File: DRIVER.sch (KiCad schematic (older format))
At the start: 24 parts, among them P1 PWR_IN, P2 HALL, P3 MOT, U1 MCT8316ZR

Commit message: Update
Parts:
- added D1: ORANGE, symbol device:LED
- added D2: BLUE, symbol device:LED
- added D3: GREEN, symbol device:LED
- added D4: RED, symbol device:LED
- added R1, R2: 1k, Resistor_SMD:R_0603_1608Metric, symbol device:R
- added R3: 4.7k, Resistor_SMD:R_0402_1005Metric, symbol device:R
- added R4: 330, Resistor_SMD:R_0402_1005Metric, symbol device:R
- R10: renamed from R6; value 10k 1% 1/16W -> 10k
- R12: renamed from R8; value 10k 1% 1/16W -> 10k
- R7: renamed from R3; value 10k 1% 1/16W -> 10k
- renumbered R7 to R11, R9 to R13, R1 to R5, R2 to R6, R4 to R8, R5 to R9
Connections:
- net labels added: +3.3V, +5V
- net labels removed: VCC, VDD
- wire segments 150 -> 167

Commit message: Update
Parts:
- C1: symbol device:CP1 -> Driverino-rescue:CP1-device
- C10, C2, C3, C4, C5, C6, C7, C8, C9: symbol device:C -> Driverino-rescue:C-device
- D1, D2, D3, D4: symbol device:LED -> Driverino-rescue:LED-device
- L1: symbol device:INDUCTOR_SMALL -> Driverino-rescue:INDUCTOR_SMALL-device
- P1: symbol conn:CONN_2 -> Driverino-rescue:CONN_2-conn
- P2: symbol conn:CONN_8 -> Driverino-rescue:CONN_8-conn
- P3: symbol conn:CONN_3 -> Driverino-rescue:CONN_3-conn
- R1, R10, R11, R12, R13, R2, R3, R4, R5, R6, R7, R8, R9: symbol device:R -> Driverino-rescue:R-device
- U1: symbol texas2:MCT8316Z -> Driverino-rescue:MCT8316Z-texas2
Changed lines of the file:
@@
 W
 $Comp
-L device:C C?
+L Driverino-rescue:C-device C?
 U 1 1 613F2407
 P 7025 4250
@@
 $EndComp
 $Comp
-L device:C C?
+L Driverino-rescue:C-device C?
 U 1 1 613F240F
 P 7025 3725
@@
 HBP
 $Comp
-L device:C C?
+L Driverino-rescue:C-device C?
 U 1 1 613F2422
 P 2250 4275
@@
 $EndComp
 $Comp
-L power:GNDPWR #PWR?
+L Driverino-rescue:GNDPWR-power #PWR?
 U 1 1 613F2428
 P 4500 5625
@@
 	6050 3600 6050 4450
 $Comp
-L device:C C?
+L Driverino-rescue:C-device C?
 U 1 1 613F2449
 P 3250 3600
@@
 	5875 3700 5875 2650
 $Comp
-L device:C C?
+L Driverino-rescue:C-device C?
 U 1 1 613F2468
 P 5875 4000
@@
 	5875 4200 5875 4450
 $Comp
-L power:GND #PWR?
+L Driverino-rescue:GND-power #PWR?
 U 1 1 613F2471
 P 5875 4650
@@
 	5500 3900 5500 4800
 $Comp
-L device:R R?
+L Driverino-rescue:R-device R?
 U 1 1 613F2482
 P 4000 1925
@@
 	4000 1575 4000 1675
 $Comp
-L device:C C?
+L Driverino-rescue:C-device C?
 U 1 1 613F2491
 P 2650 4275
@@
 	6675 3400 7025 3400
 $Comp
-L device:C C?
+L Driverino-rescue:C-device C?
 U 1 1 613F24A8
 P 7025 3200
@@
 	2250 3550 2250 3700
 $Comp
-L device:C C?
+L Driverino-rescue:C-device C?
 U 1 1 613F24BD
 P 2650 3700
@@
 Connection ~ 4700 2350
 $Comp
-L device:R R?
+L Driverino-rescue:R-device R?
 U 1 1 613F24EA
 P 4700 1925
@@
 	10325 5675 9950 5675
 $Comp
-L conn:CONN_3 P?
+L Driverino-rescue:CONN_3-conn P?
 U 1 1 614094B0
 P 10675 5575
@@
 	9375 3875 9125 3875
 $Comp
-L device:R R?
+L Driverino-rescue:R-device R?
 U 1 1 614094E1
 P 9375 4200
@@
 $EndComp
 $Comp
-L device:R R?
+L Driverino-rescue:R-device R?
 U 1 1 614094E7
 P 9550 4200
@@
 $EndComp
 $Comp
-L device:R R?
+L Driverino-rescue:R-device R?
 U 1 1 614094ED
 P 9725 4200
@@
 	9725 3375 9125 3375
 $Comp
-L device:R R?
+L Driverino-rescue:R-device R?
 U 1 1 61409506
 P 9725 3025
@@
 $EndComp
 $Comp
-L device:R R?
+L Driverino-rescue:R-device R?
 U 1 1 61409516
 P 9550 3025
@@
 $EndComp
 $Comp
-L device:R R?
+L Driverino-rescue:R-device R?
 U 1 1 61409526
 P 9375 3025
@@
 	9675 1100 9975 1100
 $Comp
-L conn:CONN_2 P?
+L Driverino-rescue:CONN_2-conn P?
 U 1 1 614328C9
 P 10675 1200
@@
 	9975 1100 10325 1100
 $Comp
-L power:GNDPWR #PWR?
+L Driverino-rescue:GNDPWR-power #PWR?
 U 1 1 614328D8
 P 9975 1500
@@
 Connection ~ 9975 1300
 $Comp
-L device:R R?
+L Driverino-rescue:R-device R?
 U 1 1 614328E5
 P 9500 1300
@@
 	9075 1300 9075 1500
 $Comp
-L power:GND #PWR?
+L Driverino-rescue:GND-power #PWR?
 U 1 1 614328EC
 P 9075 1500
@@
 MISO
 $Comp
-L device:INDUCTOR_SMALL L?
+L Driverino-rescue:INDUCTOR_SMALL-device L?
 U 1 1 6145D79B
 P 4625 6450
@@
 $EndComp
 $Comp
-L device:C C?
+L Driverino-rescue:C-device C?
 U 1 1 6145D7A1
-P 4200 6775
+P 4200 6750
 AR Path="/6145D7A1" Ref="C?"  Part="1"
 AR Path="/613CDDB7/6145D7A1" Ref="C6"  Part="1"
-F 0 "C6" H 4075 6725 40  0000 R CNN
-F 1 "22uF" H 4075 6775 40  0000 R CNN
-F 2 "" H 4238 6625 30  0000 C CNN
-F 3 "" H 4200 6775 60  0000 C CNN
-	1    4200 6775
+F 0 "C6" H 4075 6700 40  0000 R CNN
+F 1 "22uF" H 4075 6750 40  0000 R CNN
+F 2 "" H 4238 6600 30  0000 C CNN
+F 3 "" H 4200 6750 60  0000 C CNN
+	1    4200 6750
 	-1   0    0    1
 $EndComp
@@
 	4375 6450 4200 6450
 Wire Wire Line
-	4200 6450 4200 6575
-$Comp
-L power:GND #PWR?
+	4200 6450 4200 6550
+$Comp
+L Driverino-rescue:GND-power #PWR?
 U 1 1 6145D7AB
 P 4200 7125
@@
 $EndComp
 Wire Wire Line
-	4200 6975 4200 7050
+	4200 6950 4200 7050
 Wire Wire Line
 	4200 7050 5050 7050
@@
 	1625 4475 1625 4550
 $Comp
-L power:GNDPWR #PWR?
+L Driverino-rescue:GNDPWR-power #PWR?
 U 1 1 613F24DF
 P 1625 4650
@@
 	2250 4000 1625 4000
 $Comp
-L device:CP1 C?
+L Driverino-rescue:CP1-device C?
 U 1 1 613F24D7
 P 1625 4275
@@
 $EndComp
 $Comp
-L power:+5V #PWR012
+L Driverino-rescue:+5V-power #PWR012
 U 1 1 608D548F
 P 4200 6200
@@
 $EndComp
 $Comp
-L power:+3.3V #PWR016
+L Driverino-rescue:+3.3V-power #PWR016
 U 1 1 608D6090
 P 5875 2650
@@
 $EndComp
 $Comp
-L power:+3.3V #PWR011
+L Driverino-rescue:+3.3V-power #PWR011
 U 1 1 608E3D65
 P 4000 1575
@@
 $EndComp
 $Comp
-L power:+3.3V #PWR015
+L Driverino-rescue:+3.3V-power #PWR015
 U 1 1 608E3F5E
 P 4700 1575
@@
 	4000 2325 4000 2450
 $Comp
-L texas2:MCT8316Z U?
+L Driverino-rescue:MCT8316Z-texas2 U?
 U 1 1 613F23CB
 P 4350 3550
@@
 	2950 2750 2700 2750
 $Comp
-L power:GND #PWR?
+L Driverino-rescue:GND-power #PWR?
 U 1 1 613F23E8
 P 2700 2750
@@
 Connection ~ 2950 2750
 $Comp
-L power:+3.3V #PWR021
+L Driverino-rescue:+3.3V-power #PWR021
 U 1 1 609B9EEF
 P 9975 2550
@@
 	10325 3875 9375 3875
 $Comp
-L conn:CONN_8 P?
+L Driverino-rescue:CONN_8-conn P?
 U 1 1 614094BA
 P 10675 3625
@@
 	10325 3975 9975 3975
 $Comp
-L power:GND #PWR?
+L Driverino-rescue:GND-power #PWR?
 U 1 1 614094C1
 P 9975 4700
@@
 $EndComp
 $Comp
-L device:R R?
+L Driverino-rescue:R-device R?
 U 1 1 60AF5785
 P 2025 6600
@@
 $EndComp
 $Comp
-L power:GNDPWR #PWR?
+L Driverino-rescue:GNDPWR-power #PWR?
 U 1 1 60AF5F0E
 P 2025 7425
@@
 	2025 6850 2025 6900
 $Comp
-L device:LED D3
+L Driverino-rescue:LED-device D3
 U 1 1 60B03561
 P 2025 7100
@@
 	2025 7300 2025 7425
 $Comp
-L device:R R?
+L Driverino-rescue:R-device R?
 U 1 1 60B112DD
 P 2425 6600
@@
 	2425 6850 2425 6900
 $Comp
-L device:LED D4
+L Driverino-rescue:LED-device D4
 U 1 1 60B112F3
 P 2425 7100
@@
 	2425 7300 2425 7425
 $Comp
-L power:+3.3V #PWR09
+L Driverino-rescue:+3.3V-power #PWR09
 U 1 1 60B18E8B
 P 2425 6200
@@
 	2425 6200 2425 6350
 $Comp
-L device:R R?
+L Driverino-rescue:R-device R?
 U 1 1 60B5A3E5
 P 1525 6600
@@
 	1525 7300 1525 7425
 $Comp
-L power:GND #PWR?
+L Driverino-rescue:GND-power #PWR?
 U 1 1 60B5A3ED
 P 1525 7425
@@
 $EndComp
 $Comp
-L device:LED D?
+L Driverino-rescue:LED-device D?
 U 1 1 60B5A3F3
 P 1525 7100
@@
 	1525 6850 1525 6900
 $Comp
-L power:+5V #PWR?
+L Driverino-rescue:+5V-power #PWR?
 U 1 1 60B5A3FA
 P 1525 6200
@@
 $EndComp
 $Comp
-L device:R R?
+L Driverino-rescue:R-device R?
 U 1 1 60B5A406
 P 1050 6600
@@
 	1050 7300 1050 7425
 $Comp
-L power:GND #PWR?
+L Driverino-rescue:GND-power #PWR?
 U 1 1 60B5A40E
 P 1050 7425
@@
 $EndComp
 $Comp
-L device:LED D?
+L Driverino-rescue:LED-device D?
 U 1 1 60B5A414
 P 1050 7100
@@
 	1050 6850 1050 6900
 $Comp
-L power:+3.3V #PWR?
+L Driverino-rescue:+3.3V-power #PWR?
 U 1 1 60B5A41B
 P 1050 6200

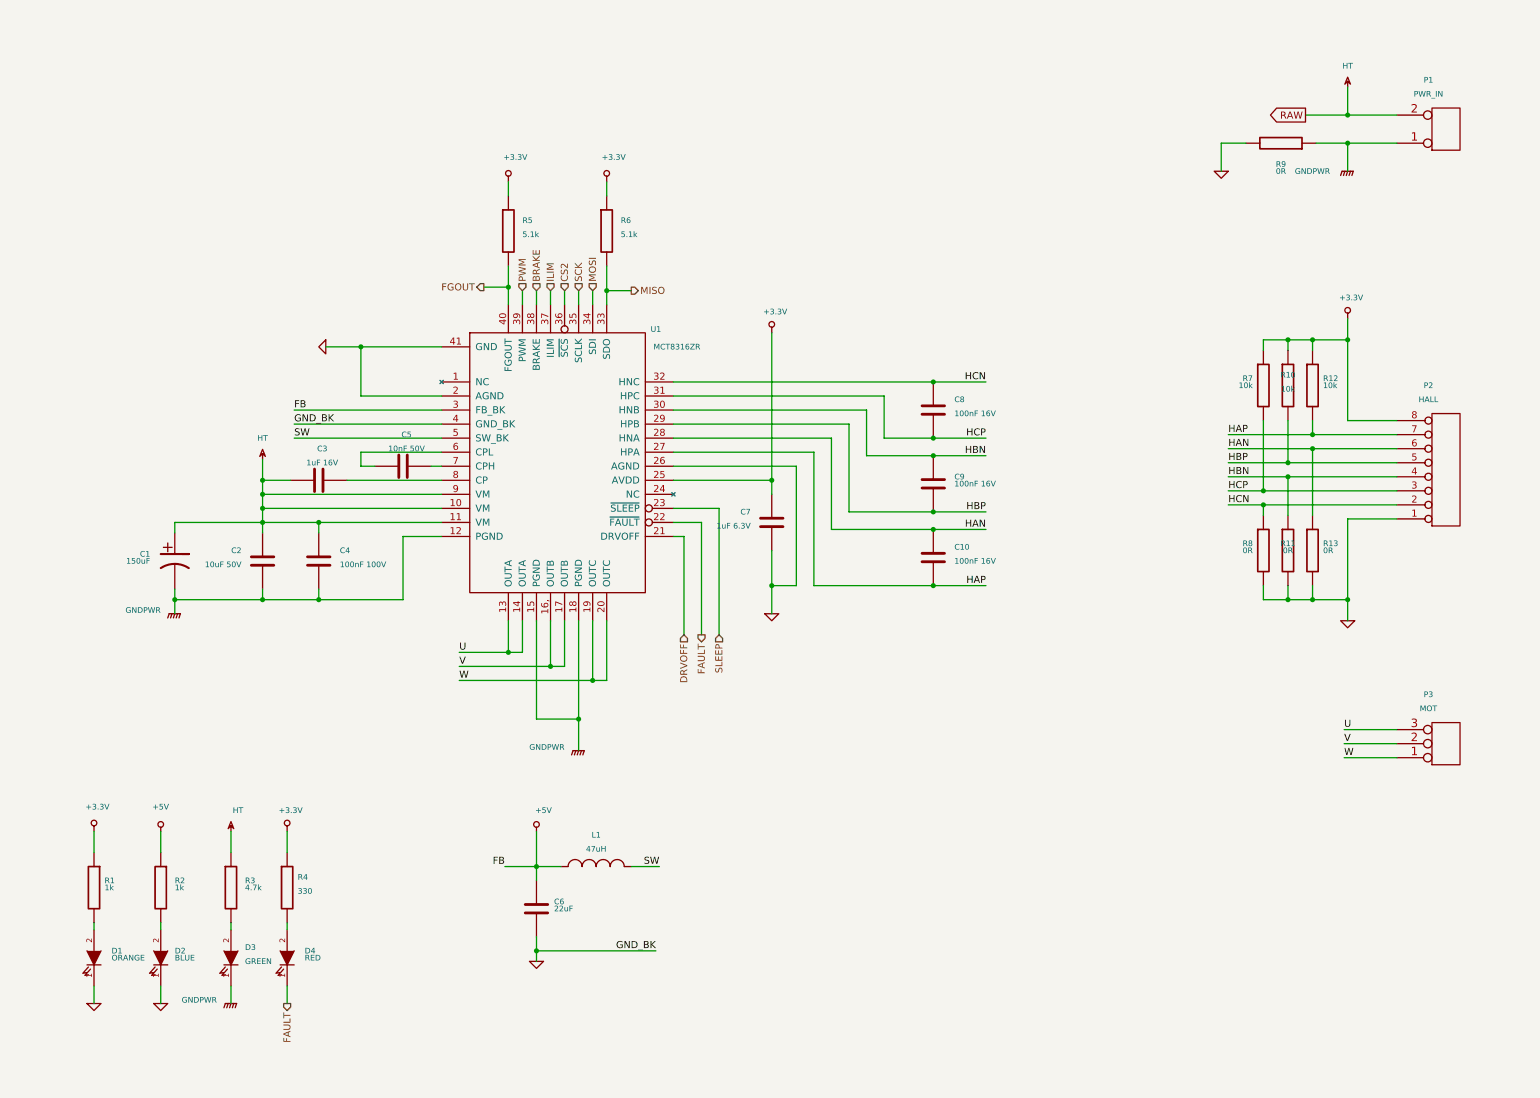
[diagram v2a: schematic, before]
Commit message: Update
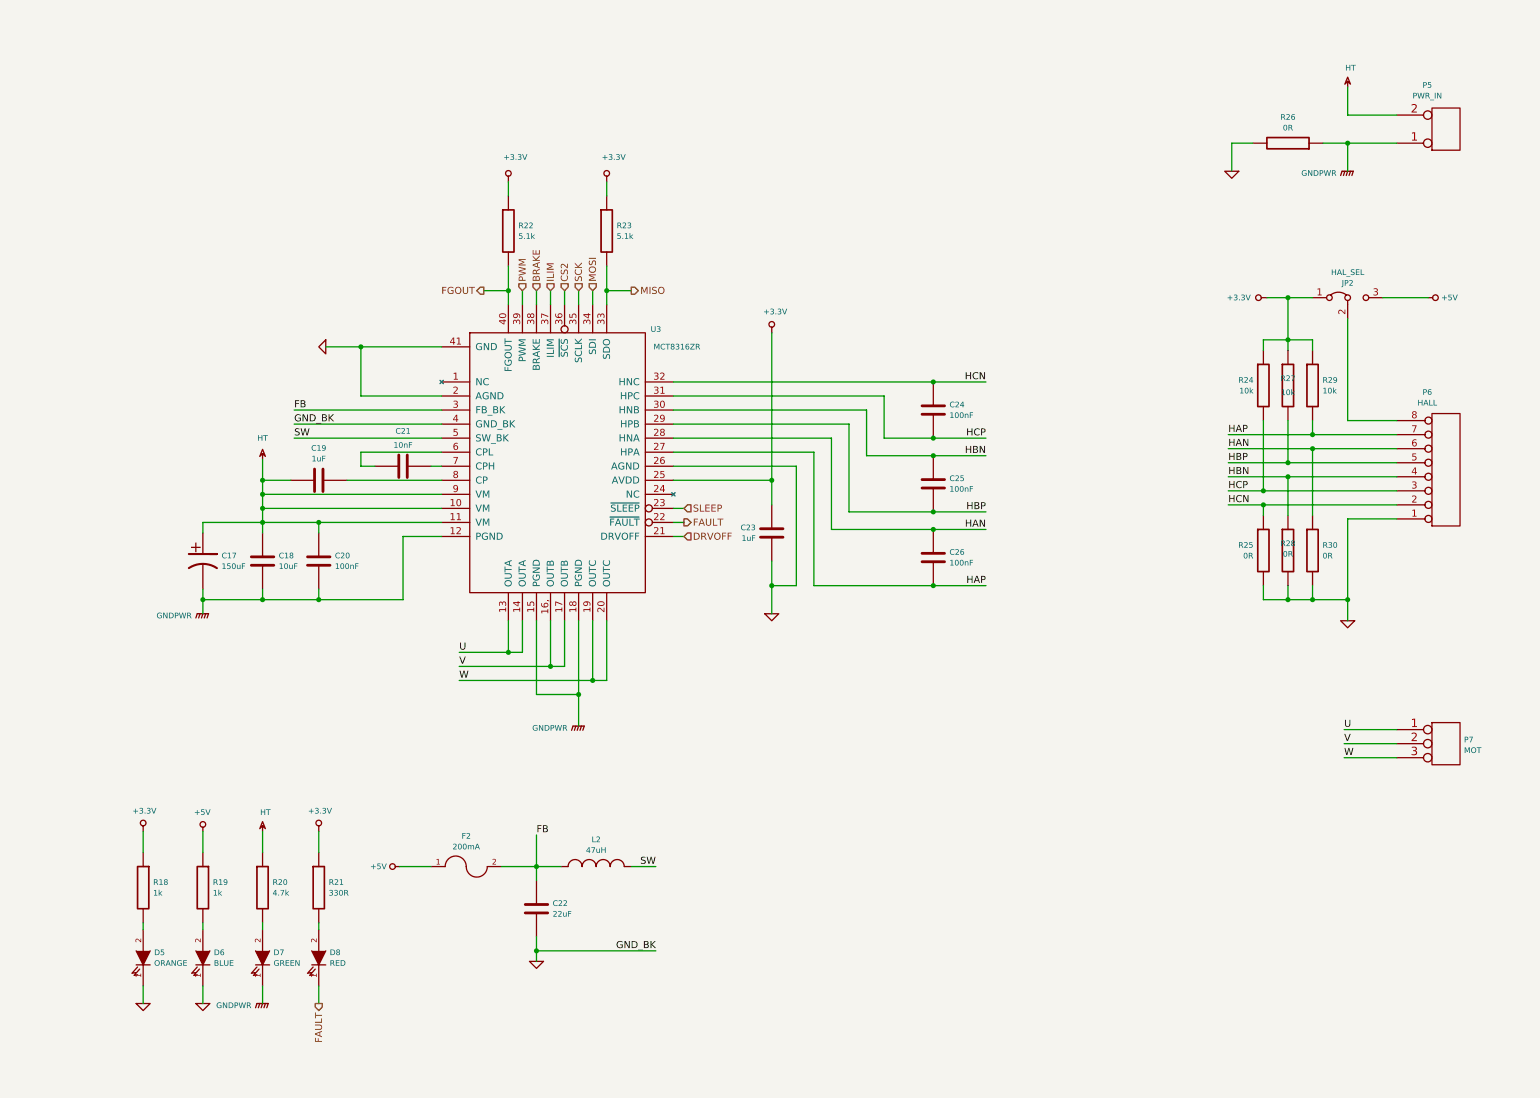
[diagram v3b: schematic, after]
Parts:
- added F2: 200mA, Fuse:Fuse_0402_1005Metric, symbol Driverino-rescue:FUSE-device
- added JP2: HAL_SEL, Driverino:TDD01H0SB1R, symbol Jumper:Jumper_3_Bridged12
- C17: renamed from C1; footprint (none) -> Capacitor_SMD:CP_Elec_6.3x7.7; P/N EEE-FTV151XAV -> (none); Productor Panasonic -> (none); Provider (none) -> Mouser; ProviderCode (none) -> 667-EEE-FTV151XAV
- C18: renamed from C2; value 10uF 50V -> 10uF; footprint Capacitor_SMD:C_0603_1608Metric -> Capacitor_SMD:C_1206_3216Metric; Manufacturer (none) -> TDK; Provider (none) -> Mouser; ProviderCode (none) -> 810-C3216X7R1H106160; manf# (none) -> C3216X7R1H106K160AE
- C19: renamed from C3; value 1uF 16V -> 1uF; Manufacturer (none) -> AVX; Provider (none) -> Mouser; ProviderCode (none) -> 581-0603DC105MAT2A; manf# (none) -> 0603DC105MAT2A
- C20: renamed from C4; value 100nF 100V -> 100nF; footprint Capacitor_SMD:C_0603_1608Metric -> Capacitor_SMD:C_0402_1005Metric; Manufacturer (none) -> Murata; Provider (none) -> Mouser; ProviderCode (none) -> 81-GCM155R71H104KE2J; manf# (none) -> GCM155R71H104KE02J
- C21: renamed from C5; value 10nF 50V -> 10nF; footprint Capacitor_SMD:C_0603_1608Metric -> Capacitor_SMD:C_0402_1005Metric; Manufacturer (none) -> Murata; Provider (none) -> Mouser; ProviderCode (none) -> 81-GRM155R71H103JA8D; manf# (none) -> GRM155R71H103JA88D
- C22: renamed from C6; footprint (none) -> Capacitor_SMD:C_1206_3216Metric; Manufacturer (none) -> Murata; Provider (none) -> Mouser; ProviderCode (none) -> 81-GCM31CR70J226KE3L; manf# (none) -> GCM31CR70J226KE23L
- C23: renamed from C7; value 1uF 6.3V -> 1uF; Manufacturer (none) -> AVX; Provider (none) -> Mouser; ProviderCode (none) -> 581-0603DC105MAT2A; manf# (none) -> 0603DC105MAT2A
- C24: renamed from C8; value 100nF 16V -> 100nF; footprint Capacitor_SMD:C_0603_1608Metric -> Capacitor_SMD:C_0402_1005Metric; Manufacturer (none) -> Murata; Provider (none) -> Mouser; ProviderCode (none) -> 81-GCM155R71H104KE2J; manf# (none) -> GCM155R71H104KE02J
- C25: renamed from C9; value 100nF 16V -> 100nF; footprint Capacitor_SMD:C_0603_1608Metric -> Capacitor_SMD:C_0402_1005Metric; Manufacturer (none) -> Murata; Provider (none) -> Mouser; ProviderCode (none) -> 81-GCM155R71H104KE2J; manf# (none) -> GCM155R71H104KE02J
- C26: renamed from C10; value 100nF 16V -> 100nF; footprint Capacitor_SMD:C_0603_1608Metric -> Capacitor_SMD:C_0402_1005Metric; Manufacturer (none) -> Murata; Provider (none) -> Mouser; ProviderCode (none) -> 81-GCM155R71H104KE2J; manf# (none) -> GCM155R71H104KE02J
- D5: renamed from D1; footprint (none) -> LED_SMD:LED_0603_1608Metric; Manufacturer (none) -> Kingbright; Provider (none) -> Mouser; ProviderCode (none) -> 604-AP1608SECK; manf# (none) -> AP1608SECK
- D6: renamed from D2; footprint (none) -> LED_SMD:LED_0603_1608Metric; Manufacturer (none) -> Kingbright; Provider (none) -> Mouser; ProviderCode (none) -> 604-APT1608QBC/D; manf# (none) -> APT1608QBC/D
- D7: renamed from D3; footprint (none) -> LED_SMD:LED_0603_1608Metric; Manufacturer (none) -> Kingbright; Provider (none) -> Mouser; ProviderCode (none) -> 604-APT1608SGC; manf# (none) -> APT1608SGC
- D8: renamed from D4; footprint (none) -> LED_SMD:LED_0603_1608Metric; Manufacturer (none) -> Kingbright; Provider (none) -> Mouser; ProviderCode (none) -> 604-APT1608EC; manf# (none) -> APT1608EC
- L2: renamed from L1; footprint (none) -> Inductor_SMD:L_1210_3225Metric; Manufacturer (none) -> Taiyo Yuden; Provider (none) -> Mouser; ProviderCode (none) -> 963-CBC3225T470KRV; manf# (none) -> CBC3225T470KRV
- P5: renamed from P1; footprint (none) -> Driverino:39773-0002; P/N 397730002 -> (none); Productor Molex -> (none); Provider (none) -> Mouser; ProviderCode (none) -> 538-39773-0002; manf# 397730002 -> 39773-0002
- P6: renamed from P2; footprint Connector_Molex:Molex_PicoBlade_53047-0810_1x03_P1.25mm_Vertical -> Connector_Molex:Molex_PicoBlade_53047-0810_1x08_P1.25mm_Vertical; Productor Molex -> (none); Provider (none) -> Mouser; ProviderCode (none) -> 538-53047-0810
- P7: renamed from P3; footprint (none) -> Driverino:39773-0003; P/N 397730003 -> (none); Productor Molex -> (none); Provider (none) -> Mouser; ProviderCode (none) -> 538-39773-0003; manf# 397730003 -> 39773-0003
- R18: renamed from R1; footprint Resistor_SMD:R_0603_1608Metric -> Resistor_SMD:R_0402_1005Metric; Manufacturer (none) -> Vishay; P/N CRCW0603332RFKEA -> (none); Productor Vishay -> (none); Provider (none) -> Mouser; ProviderCode (none) -> 71-CRCW04021K00FKEDC; manf# (none) -> CRCW04021K00FKEDC
- R19: renamed from R2; footprint Resistor_SMD:R_0603_1608Metric -> Resistor_SMD:R_0402_1005Metric; Manufacturer (none) -> Vishay; P/N CRCW0603332RFKEA -> (none); Productor Vishay -> (none); Provider (none) -> Mouser; ProviderCode (none) -> 71-CRCW04021K00FKEDC; manf# (none) -> CRCW04021K00FKEDC
- R20: renamed from R3; Manufacturer (none) -> Yageo; Productor TE Connectivity -> (none); Provider (none) -> Mouser; ProviderCode (none) -> 603-RC0402FR-074K7L; manf# (none) -> RC0402FR-074K7L
- R21: renamed from R4; value 330 -> 330R; Manufacturer (none) -> Vishay; Productor TE Connectivity -> (none); Provider (none) -> Mouser; ProviderCode (none) -> 756-GWCR0402330RFT10; manf# (none) -> CRCW0402330RFKED
- R22: renamed from R5; Manufacturer (none) -> ROHM; Provider (none) -> Mouser; ProviderCode (none) -> 755-SFR01MZPF5101; manf# (none) -> SFR01MZPF5101
- R23: renamed from R6; Manufacturer (none) -> ROHM; Provider (none) -> Mouser; ProviderCode (none) -> 755-SFR01MZPF5101; manf# (none) -> SFR01MZPF5101
- R24: renamed from R7; Manufacturer (none) -> Vishay; Productor TE Connectivity -> (none); Provider (none) -> Mouser; ProviderCode (none) -> 71-CRCW040210K0FKEDC; manf# (none) -> CRCW040210K0FKEDC
- R25: renamed from R8; footprint Resistor_SMD:R_0603_1608Metric -> Resistor_SMD:R_0402_1005Metric; Manufacturer (none) -> Vishay; Provider (none) -> Mouser; ProviderCode (none) -> 71-RCC04020000Z0ED; manf# (none) -> RCC04020000Z0ED
- R26: renamed from R9; footprint Resistor_SMD:R_0603_1608Metric -> Resistor_SMD:R_0402_1005Metric; Manufacturer (none) -> Vishay; P/N ERJU03F22R0V -> (none); Provider (none) -> Mouser; ProviderCode (none) -> 71-RCC04020000Z0ED; manf# (none) -> RCC04020000Z0ED
- R27: renamed from R10; Manufacturer (none) -> Vishay; Productor TE Connectivity -> (none); Provider (none) -> Mouser; ProviderCode (none) -> 71-CRCW040210K0FKEDC; manf# (none) -> CRCW040210K0FKEDC
- R28: renamed from R11; footprint Resistor_SMD:R_0603_1608Metric -> Resistor_SMD:R_0402_1005Metric; Manufacturer (none) -> Vishay; Provider (none) -> Mouser; ProviderCode (none) -> 71-RCC04020000Z0ED; manf# (none) -> RCC04020000Z0ED
- R29: renamed from R12; Manufacturer (none) -> Vishay; Productor TE Connectivity -> (none); Provider (none) -> Mouser; ProviderCode (none) -> 71-CRCW040210K0FKEDC; manf# (none) -> CRCW040210K0FKEDC
- R30: renamed from R13; footprint Resistor_SMD:R_0603_1608Metric -> Resistor_SMD:R_0402_1005Metric; Manufacturer (none) -> Vishay; Provider (none) -> Mouser; ProviderCode (none) -> 71-RCC04020000Z0ED; manf# (none) -> RCC04020000Z0ED
- U3: renamed from U1; footprint (none) -> Driverino:QFN-40_EP_5x7_Pitch0.5mm; Productor TI -> (none)
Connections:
- net +3.3V: now also JP2.1 (A); no longer P6.8 (P8)
- net +5V: now also F2.1, JP2.3 (B); no longer C22.2, L2.2, U3.3 (FB_BK)
- net U: now also P7.1 (P1); no longer P7.3 (P3)
- net W: now also P7.3 (P3); no longer P7.1 (P1)
- new net: JP2.2 (C), P6.8 (P8)
- new net FB: C22.2, F2.2, L2.2, U3.3 (FB_BK)
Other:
- moved on the sheet: C17, C23, D5, D6, D7, D8, R18, R19, R20, R21, R26

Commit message: Update
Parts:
- JP2: symbol Jumper:Jumper_3_Bridged12 -> Driverino-rescue:Jumper_3_Bridged12-Jumper
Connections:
- net GNDPWR: now also P5.2 (PM); no longer P5.1 (P1)
- net HT: now also P5.1 (P1); no longer P5.2 (PM)
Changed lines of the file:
@@
 AR Path="/614328C9" Ref="P?"  Part="1"
 AR Path="/613CDDB7/614328C9" Ref="P5"  Part="1"
-F 0 "P5" H 10542 887 40  0000 C CNN
-F 1 "PWR_IN" H 10542 963 40  0000 C CNN
+F 0 "P5" H 10850 1250 40  0000 L CNN
+F 1 "PWR_IN" H 10850 1150 40  0000 L CNN
 F 2 "Driverino:39773-0002" H 10675 1200 50  0001 C CNN
 F 3 "" H 10675 1200 50  0001 C CNN
@@
 F 9 "538-39773-0002" H 10675 1200 50  0001 C CNN "ProviderCode"
 	1    10675 1200
-	1    0    0    1
+	1    0    0    -1
 $EndComp
 $Comp
@@
 $EndComp
 $Comp
-L Jumper:Jumper_3_Bridged12 JP?
+L Driverino-rescue:Jumper_3_Bridged12-Jumper JP?
 U 1 1 6091D84F
 P 9975 2400

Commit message: Update
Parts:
- JP2: footprint Driverino:TDD01H0SB1R -> Connector_PinHeader_1.27mm:PinHeader_1x03_P1.27mm_Vertical; Manufacturer C&K -> Samtec; ProviderCode 611-TDD01H0SB1R -> 200-TMS10301GS; manf# TDD01H0SB1R -> TMS-103-01-G-S
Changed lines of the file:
@@
 F 0 "JP2" H 9975 2504 40  0000 C CNN
 F 1 "HAL_SEL" H 9975 2580 40  0000 C CNN
-F 2 "Driverino:TDD01H0SB1R" H 9975 2400 50  0001 C CNN
+F 2 "Connector_PinHeader_1.27mm:PinHeader_1x03_P1.27mm_Vertical" H 9975 2400 50  0001 C CNN
 F 3 "~" H 9975 2400 50  0001 C CNN
-F 4 "	C&K" H 9975 2400 50  0001 C CNN "Manufacturer"
+F 4 "Samtec" H 9975 2400 50  0001 C CNN "Manufacturer"
 F 5 "Mouser" H 9975 2400 50  0001 C CNN "Provider"
-F 6 "611-TDD01H0SB1R" H 9975 2400 50  0001 C CNN "ProviderCode"
-F 7 "TDD01H0SB1R" H 9975 2400 50  0001 C CNN "manf#"
+F 6 "200-TMS10301GS" H 9975 2400 50  0001 C CNN "ProviderCode"
+F 7 "TMS-103-01-G-S" H 9975 2400 50  0001 C CNN "manf#"
 	1    9975 2400
 	1    0    0    -1
